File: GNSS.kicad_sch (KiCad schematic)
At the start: 11 parts, among them U14 SAM-M10Q-00B

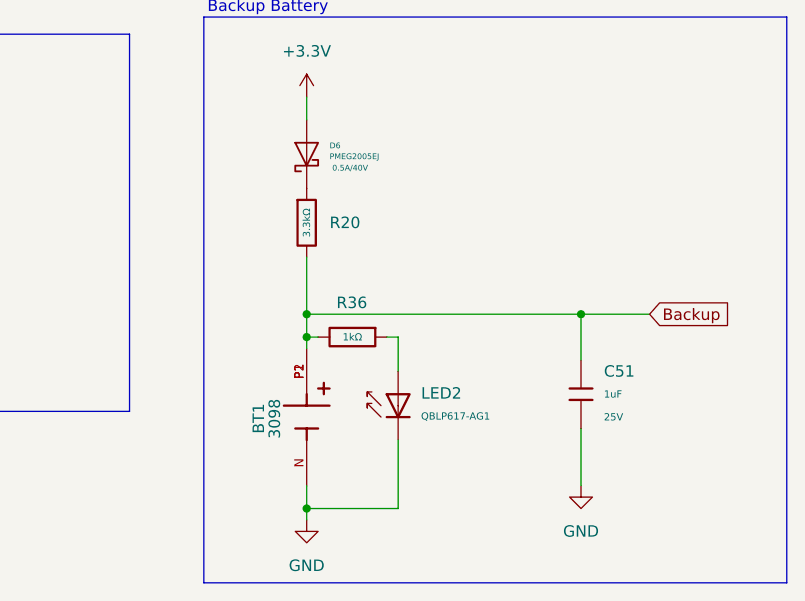
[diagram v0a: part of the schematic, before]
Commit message: Chore: push new design
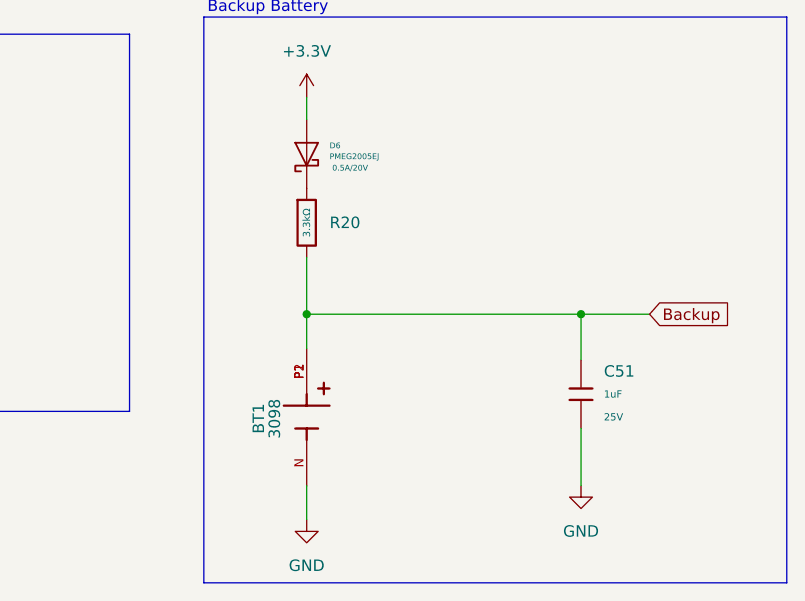
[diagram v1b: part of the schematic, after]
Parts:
- removed LED2: QBLP617-AG1, PCM_JLCPCB:D_0603, symbol PCM_JLCPCB-Diodes:LED,0603,Red
- removed R36: 1kΩ, PCM_JLCPCB:R_0603, symbol PCM_JLCPCB-Resistors:0402,1kΩ
- C51: footprint PCM_JLCPCB:C_0402 -> PCM_JLCPCB:C_0603
- D6: Ratings 0.5A/40V -> 0.5A/20V

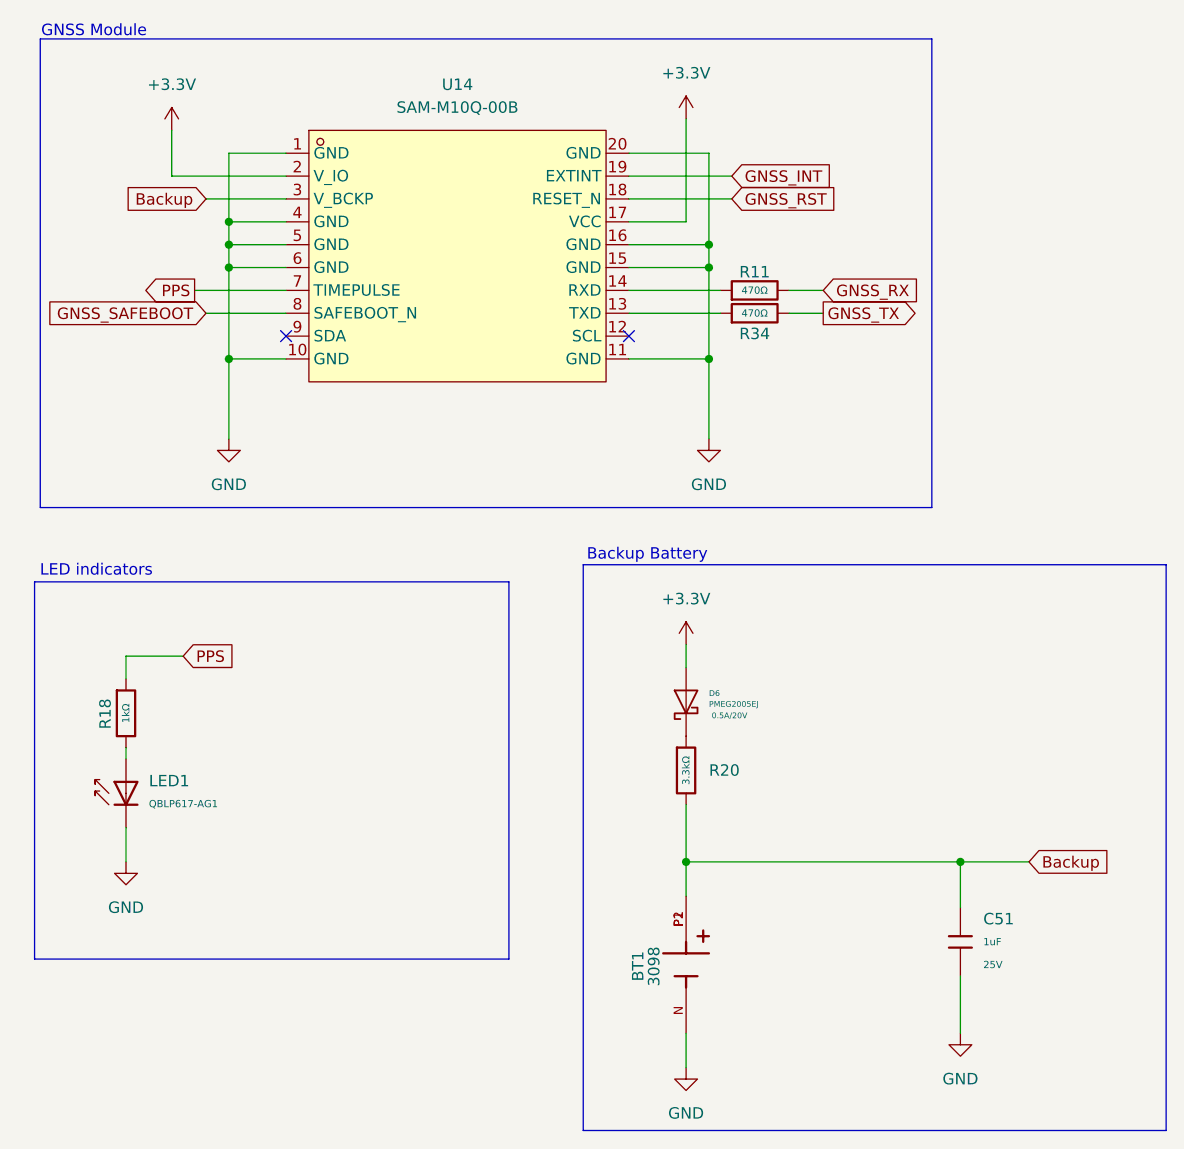
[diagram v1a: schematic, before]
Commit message: Special version
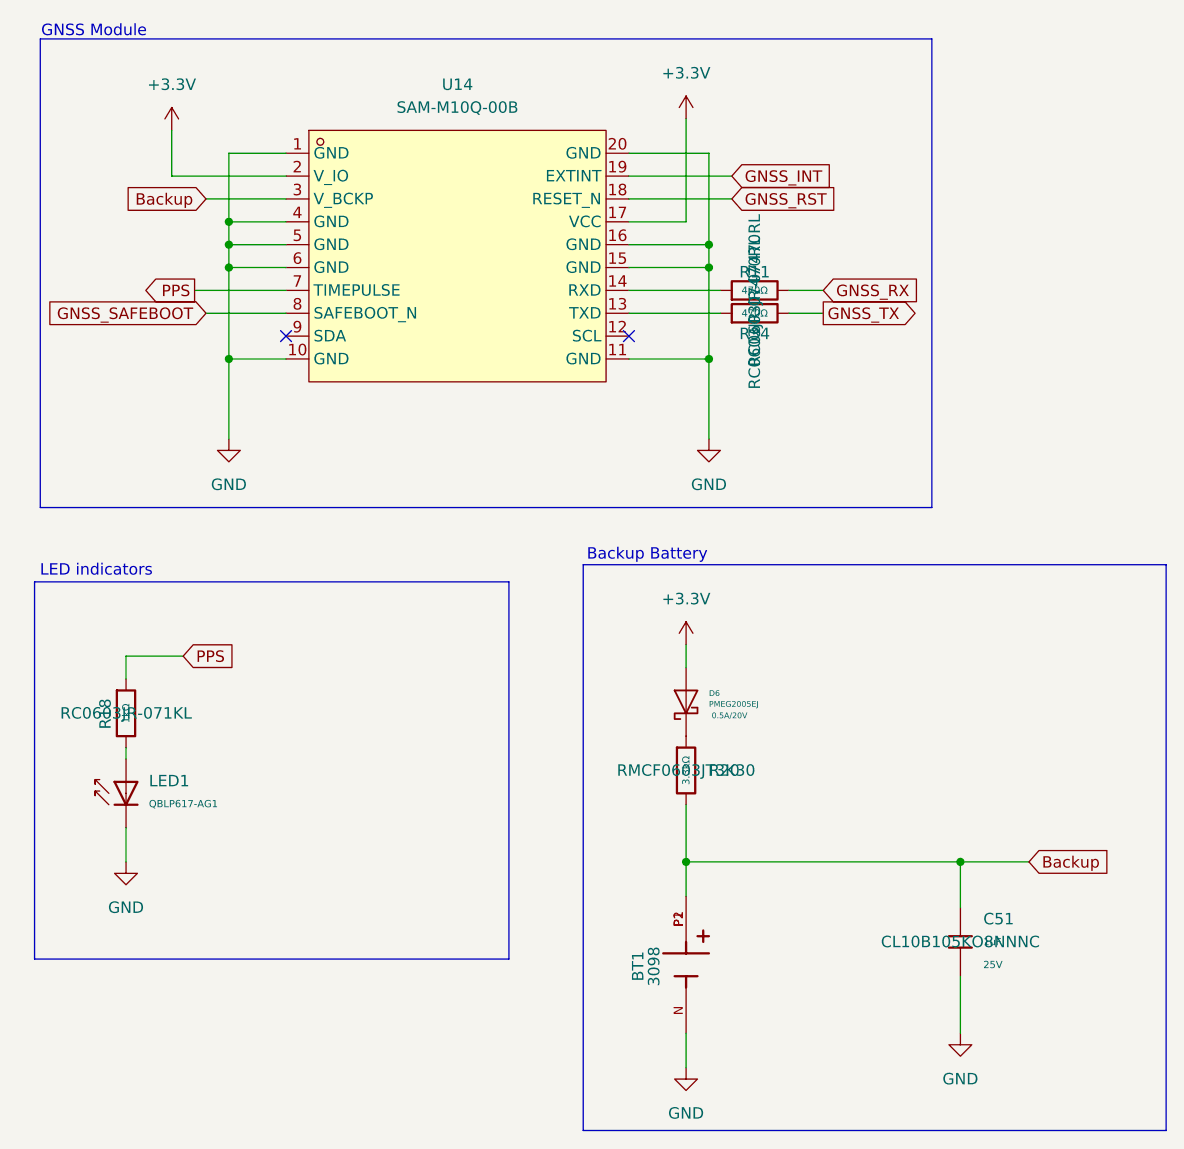
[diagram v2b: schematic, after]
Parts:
- C51: Digikey Parts (none) -> CL10B105KO8NNNC
- R11, R34: Digikey Parts (none) -> RC0603JR-07470RL
- R18: Digikey Parts (none) -> RC0603JR-071KL
- R20: Digikey Parts (none) -> RMCF0603JT3K30
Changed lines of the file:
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@@
+			)
+		)
+		(property "Digikey Parts" ""
+			(at 92.71 92.71 0)
+			(effects
+				(font
+					(size 1.27 1.27)
+				)
 			)
 		)
@@
 			)
 		)
+		(property "Digikey Parts" "RC0603JR-071KL"
+			(at 30.48 93.98 0)
+			(effects
+				(font
+					(size 1.27 1.27)
+				)
+			)
+		)
 		(pin "1"
 		)
@@
 			)
 		)
+		(property "Digikey Parts" "RMCF0603JT3K30"
+			(at 92.71 100.33 0)
+			(effects
+				(font
+					(size 1.27 1.27)
+				)
+			)
+		)
 		(pin "1"
 		)
@@
 			)
 		)
+		(property "Digikey Parts" "RC0603JR-07470RL"
+			(at 100.33 49.53 0)
+			(effects
+				(font
+					(size 1.27 1.27)
+				)
+			)
+		)
 		(pin "1"
 		)
@@
 			)
 		)
+		(property "Digikey Parts" "CL10B105KO8NNNC"
+			(at 123.19 119.38 0)
+			(effects
+				(font
+					(size 1.27 1.27)
+				)
+			)
+		)
 		(pin "2"
 		)
@@
 			)
 		)
+		(property "Digikey Parts" "RC0603JR-07470RL"
+			(at 100.33 46.99 0)
+			(effects
+				(font
+					(size 1.27 1.27)
+				)
+			)
+		)
 		(pin "1"
 		)
@@
 			)
 		)
+		(property "Digikey Parts" ""
+			(at 30.48 102.87 0)
+			(effects
+				(font
+					(size 1.27 1.27)
+				)
+			)
+		)
 		(pin "2"
 		)
@@
 			)
 		)
+		(property "Digikey Parts" ""
+			(at 67.31 43.18 0)
+			(effects
+				(font
+					(size 1.27 1.27)
+				)
+			)
+		)
 		(pin "6"
 		)
@@
 			(at 92.71 121.92 0)
 			(effects
+				(font
+					(size 1.27 1.27)
+				)
+			)
+		)
+		(property "Digikey Parts" ""
+			(at 92.71 121.92 0)
+			(effects
